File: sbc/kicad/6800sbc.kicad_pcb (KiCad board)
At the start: 2 copper layers, 147 parts, among them J1 AC/DC IN, J10 BAUD RATE, J11 SEGMENT TEST, J12 REG. POWER, J2 5V IN, J3 EXPANSION, J4 LTC, J5 Parallel Port, J6 TX DATA SELECT, J7 RX DATA SELECT, J8 USB POWER, J9 FTDI SERIAL, SW10 "9", SW11 "4", SW12 "5", SW13 "6", SW14 "1", SW15 "2", SW16 "3", SW17 "0", SW18 "RESET", SW2 "D", SW3 "E", SW4 "F", SW5 "A", SW6 "B", SW7 "C", SW8 "7", SW9 "8", U1 LM7805, U10 MAN71A, U11 MAN71A, U12 74LS259, U13 74LS259, U14 74LS259, U15 74LS259, U16 74LS259, U17 74LS259, U18 74LS244, U19 62256 RAM, U2 74LS00, U20 27128, U21 MC6802, U22 ATF16V8B, U23 74LS244, U24 74LS42, U3 74LS04, U4 6821, U5 MC6850, U6 MAN71A, U7 MAN71A, U8 MAN71A, U9 MAN71A, Y1 1.8432 MHz, Y2 3.579545 kHz

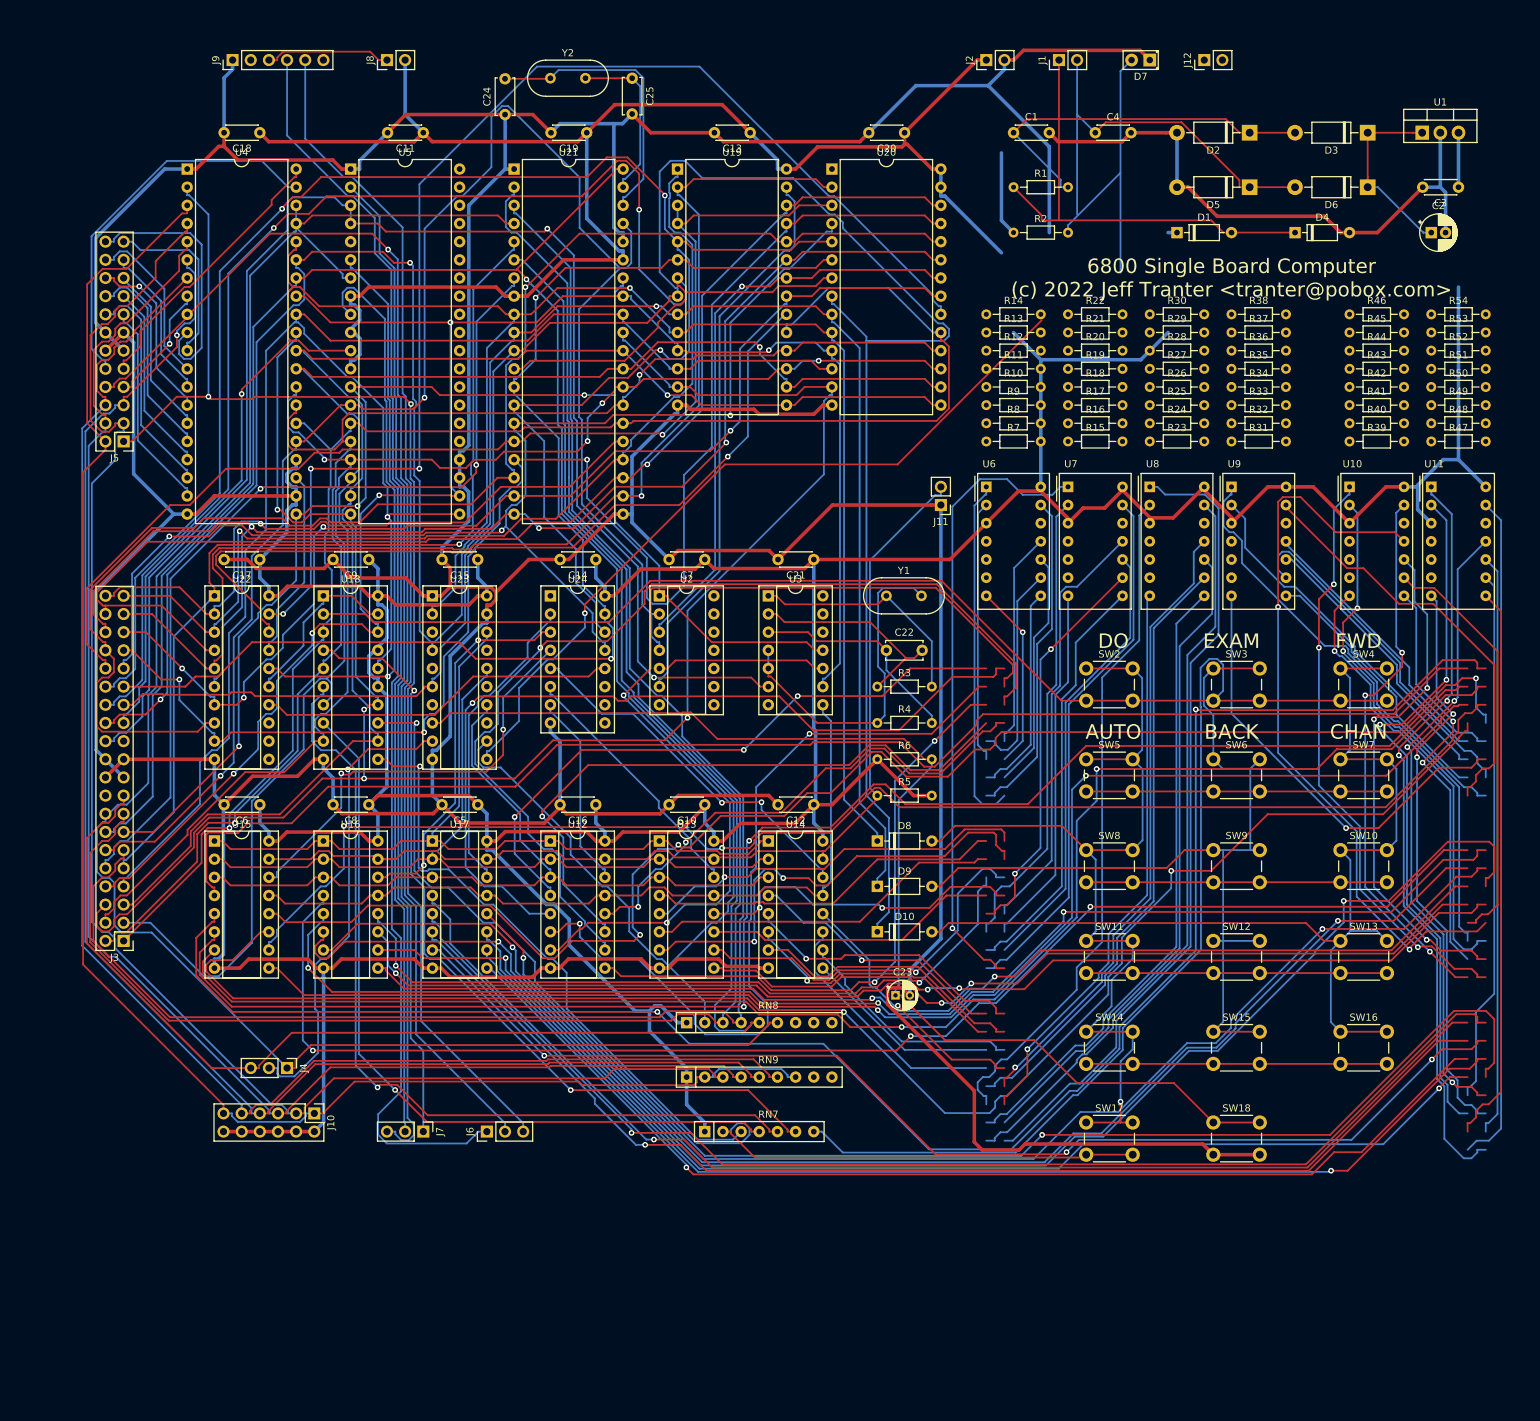
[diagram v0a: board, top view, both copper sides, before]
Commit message: Getting close to ready to order PCBs. Check in all files.
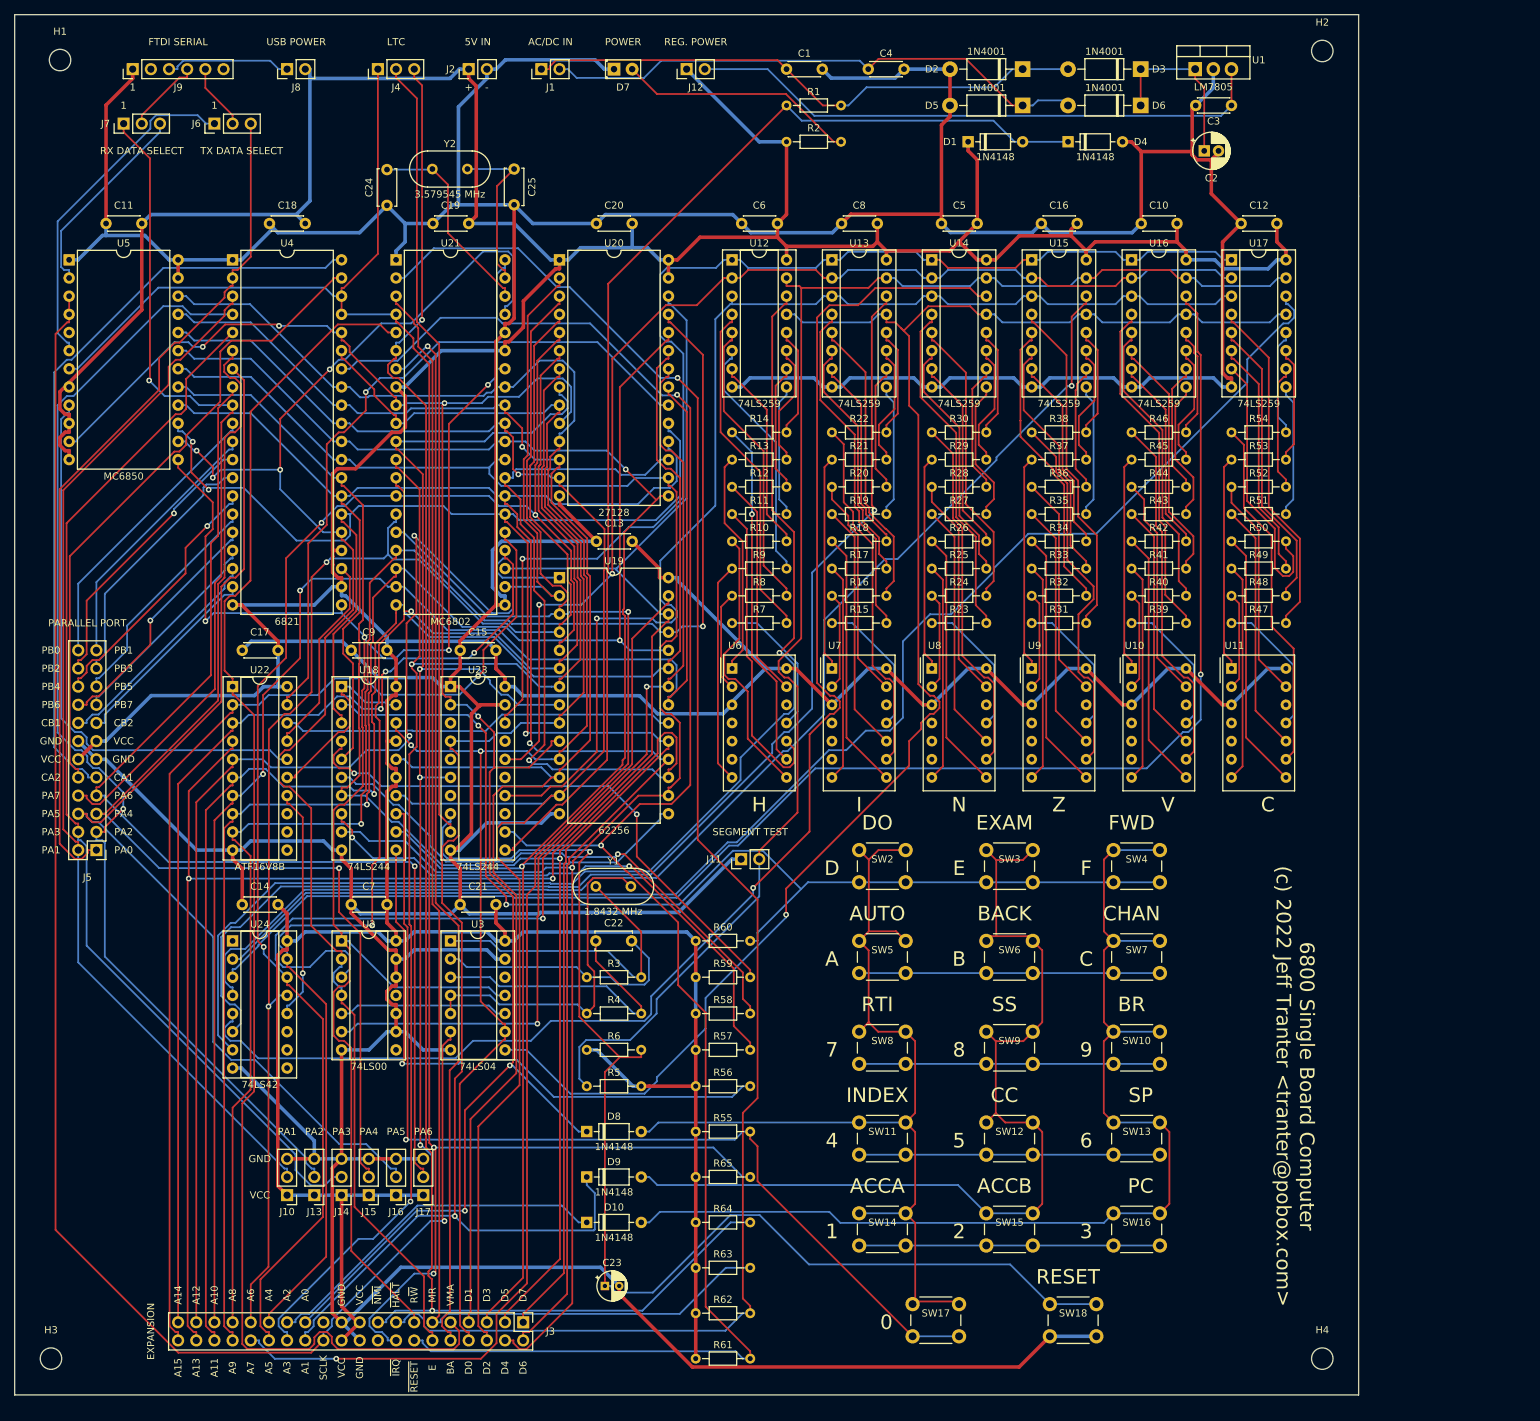
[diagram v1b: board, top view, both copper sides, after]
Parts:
- removed RN7: 8K2, Resistor_THT:R_Array_SIP7
- removed RN8, RN9: 3K, Resistor_THT:R_Array_SIP9
- added H1: MountingHole_3mm, MountingHole:MountingHole_3mm, F.Cu at (39.4, 29.2)
- added H2: MountingHole_3mm, MountingHole:MountingHole_3mm, F.Cu at (215.9, 27.9)
- added H3: MountingHole_3mm, MountingHole:MountingHole_3mm, F.Cu at (38.1, 210.8)
- added H4: MountingHole_3mm, MountingHole:MountingHole_3mm, F.Cu at (215.9, 210.8)
- added J13: PA2, Connector_PinHeader_2.54mm:PinHeader_1x03_P2.54mm_Vertical, F.Cu at (74.9, 188.0)
- added J14: PA3, Connector_PinHeader_2.54mm:PinHeader_1x03_P2.54mm_Vertical, F.Cu at (78.7, 188.0)
- added J15: PA4, Connector_PinHeader_2.54mm:PinHeader_1x03_P2.54mm_Vertical, F.Cu at (82.5, 188.0)
- added J16: PA5, Connector_PinHeader_2.54mm:PinHeader_1x03_P2.54mm_Vertical, F.Cu at (86.4, 188.0)
- added J17: PA6, Connector_PinHeader_2.54mm:PinHeader_1x03_P2.54mm_Vertical, F.Cu at (90.2, 188.0)
- added R55: 8K2, Resistor_THT:R_Axial_DIN0204_L3.6mm_D1.6mm_P7.62mm_Horizontal, F.Cu at (128.3, 179.1)
- added R56: 8K2, Resistor_THT:R_Axial_DIN0204_L3.6mm_D1.6mm_P7.62mm_Horizontal, F.Cu at (128.3, 172.7)
- added R57: 8K2, Resistor_THT:R_Axial_DIN0204_L3.6mm_D1.6mm_P7.62mm_Horizontal, F.Cu at (128.3, 167.6)
- added R58: 8K2, Resistor_THT:R_Axial_DIN0204_L3.6mm_D1.6mm_P7.62mm_Horizontal, F.Cu at (128.3, 162.6)
- added R59: 8K2, Resistor_THT:R_Axial_DIN0204_L3.6mm_D1.6mm_P7.62mm_Horizontal, F.Cu at (128.3, 157.5)
- added R60: 8K2, Resistor_THT:R_Axial_DIN0204_L3.6mm_D1.6mm_P7.62mm_Horizontal, F.Cu at (128.3, 152.4)
- added R61: 3K, Resistor_THT:R_Axial_DIN0204_L3.6mm_D1.6mm_P7.62mm_Horizontal, F.Cu at (128.3, 210.8)
- added R62: 3K, Resistor_THT:R_Axial_DIN0204_L3.6mm_D1.6mm_P7.62mm_Horizontal, F.Cu at (128.3, 204.5)
- added R63: 3K, Resistor_THT:R_Axial_DIN0204_L3.6mm_D1.6mm_P7.62mm_Horizontal, F.Cu at (128.3, 198.1)
- added R64: 3K, Resistor_THT:R_Axial_DIN0204_L3.6mm_D1.6mm_P7.62mm_Horizontal, F.Cu at (128.3, 191.8)
- added R65: 3K, Resistor_THT:R_Axial_DIN0204_L3.6mm_D1.6mm_P7.62mm_Horizontal, F.Cu at (128.3, 185.4)
- J10: value BAUD RATE -> PA1; footprint Connector_PinHeader_2.54mm:PinHeader_2x06_P2.54mm_Vertical -> Connector_PinHeader_2.54mm:PinHeader_1x03_P2.54mm_Vertical
- J5: value Parallel Port -> PARALLEL PORT
- U19: value 62256 RAM -> 62256
- U5: footprint Package_DIP:DIP-40_W15.24mm -> Package_DIP:DIP-24_W15.24mm
- Y2: value 3.579545 kHz -> 3.579545 MHz
- moved J7 147.1 mm to (48.3, 38.1), turned to 90 degrees
- moved J6 146.0 mm to (61.0, 38.1)
- moved J4 140.3 mm to (83.8, 30.5), turned to 90 degrees
- moved U15 140.3 mm to (175.3, 57.1)
- moved U16 139.2 mm to (189.2, 57.1)
- moved U17 138.2 mm to (203.2, 57.1)
- moved C6 108.8 mm to (139.7, 52.1)
- moved C8 108.0 mm to (153.7, 52.1)
- moved C5 107.2 mm to (167.6, 52.1)
- moved C16 105.5 mm to (181.6, 52.1)
- moved C10 104.7 mm to (195.6, 52.1)
- moved C12 103.9 mm to (209.6, 52.1)
- moved U12 85.2 mm to (133.3, 57.1)
- moved U13 84.8 mm to (147.3, 57.1)
- moved U14 84.4 mm to (161.3, 57.1)
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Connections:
- J10 pad 1: PA1 -> VCC
- J10 pad 2: GND -> PA1
- J10 pad 3: PA2 -> GND
- U2 pad 14: (no net) -> VCC
- U2 pad 7: (no net) -> GND
- U3 pad 14: (no net) -> VCC
- U3 pad 7: (no net) -> GND
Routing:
- net Net-(R32-Pad2): track 251.2 -> 41.5 mm, vias 2 -> 0
- net Net-(R37-Pad2): track 225.1 -> 17.2 mm, vias 2 -> 0
- net Net-(R38-Pad2): track 206.7 -> 15.5 mm, vias 3 -> 0
- net Net-(R34-Pad2): track 216.9 -> 27.5 mm, vias 2 -> 0
- net Net-(R33-Pad2): track 220.2 -> 34.7 mm, vias 2 -> 0
- net Net-(R35-Pad2): track 199.2 -> 18.6 mm, vias 2 -> 0
- net Net-(R44-Pad2): track 196.9 -> 18.3 mm, vias 2 -> 0
- net Net-(R36-Pad2): track 196.2 -> 17.9 mm, vias 3 -> 0
- net Net-(R42-Pad2): track 197.2 -> 27.4 mm, vias 2 -> 0
- net Net-(R41-Pad2): track 197.6 -> 34.7 mm, vias 2 -> 0
- net Net-(R54-Pad2): track 174.6 -> 15.1 mm, vias 2 -> 0
- net ~DISP5EN: track 52.3 -> 211.5 mm, vias 2 -> 1
- net ~DISP6EN: track 43.3 -> 198.0 mm
- net Net-(J6-Pad2): track 162.8 -> 9.20 mm
- net Net-(R46-Pad2): track 169.0 -> 15.5 mm, vias 3 -> 0
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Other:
- board outline added: 188 x 193 mm
- board text added: "+"
- board text added: "-"
- board text added: "0"
- board text added: "1"
- board text added: "2"
- board text added: "3"
- board text added: "4"
- board text added: "5"
- board text added: "6"
- board text added: "7"
- board text added: "8"
- board text added: "9"
- board text added: "A"
- board text added: "A0"
- board text added: "A1"
- board text added: "A10"
- board text added: "A11"
- board text added: "A12"
- board text added: "A13"
- board text added: "A14"
- board text added: "A15"
- board text added: "A2"
- board text added: "A3"
- board text added: "A4"
- board text added: "A5"
- board text added: "A6"
- board text added: "A7"
- board text added: "A8"
- board text added: "A9"
- board text added: "ACCA"
- board text added: "ACCB"
- board text added: "B"
- board text added: "BA"
- board text added: "BR"
- board text added: "C"
- board text added: "CA1"
- board text added: "CA2"
- board text added: "CB1"
- board text added: "CB2"
- board text added: "CC"
- board text added: "D"
- board text added: "D0"
- board text added: "D1"
- board text added: "D2"
- board text added: "D3"
- board text added: "D4"
- board text added: "D5"
- board text added: "D6"
- board text added: "D7"
- board text added: "E"
- board text added: "F"
- board text added: "GND"
- board text added: "H"
- board text added: "I"
- board text added: "INDEX"
- board text added: "MR"
- board text added: "N"
- board text added: "PA0"
- board text added: "PA1"
- board text added: "PA2"
- board text added: "PA3"
- board text added: "PA4"
- board text added: "PA5"
- board text added: "PA6"
- board text added: "PA7"
- board text added: "PB0"
- board text added: "PB1"
- board text added: "PB2"
- board text added: "PB3"
- board text added: "PB4"
- board text added: "PB5"
- board text added: "PB6"
- board text added: "PB7"
- board text added: "PC"
- board text added: "RESET"
- board text added: "RTI"
- board text added: "R~W"
- board text added: "SCLK"
- board text added: "SP"
- board text added: "SS"
- board text added: "V"
- board text added: "VCC"
- board text added: "VMA"
- board text added: "Z"
- board text added: "~HALT"
- board text added: "~IRQ"
- board text added: "~NMI"
- board text added: "~RESET"

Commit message: Optimizing board layout.
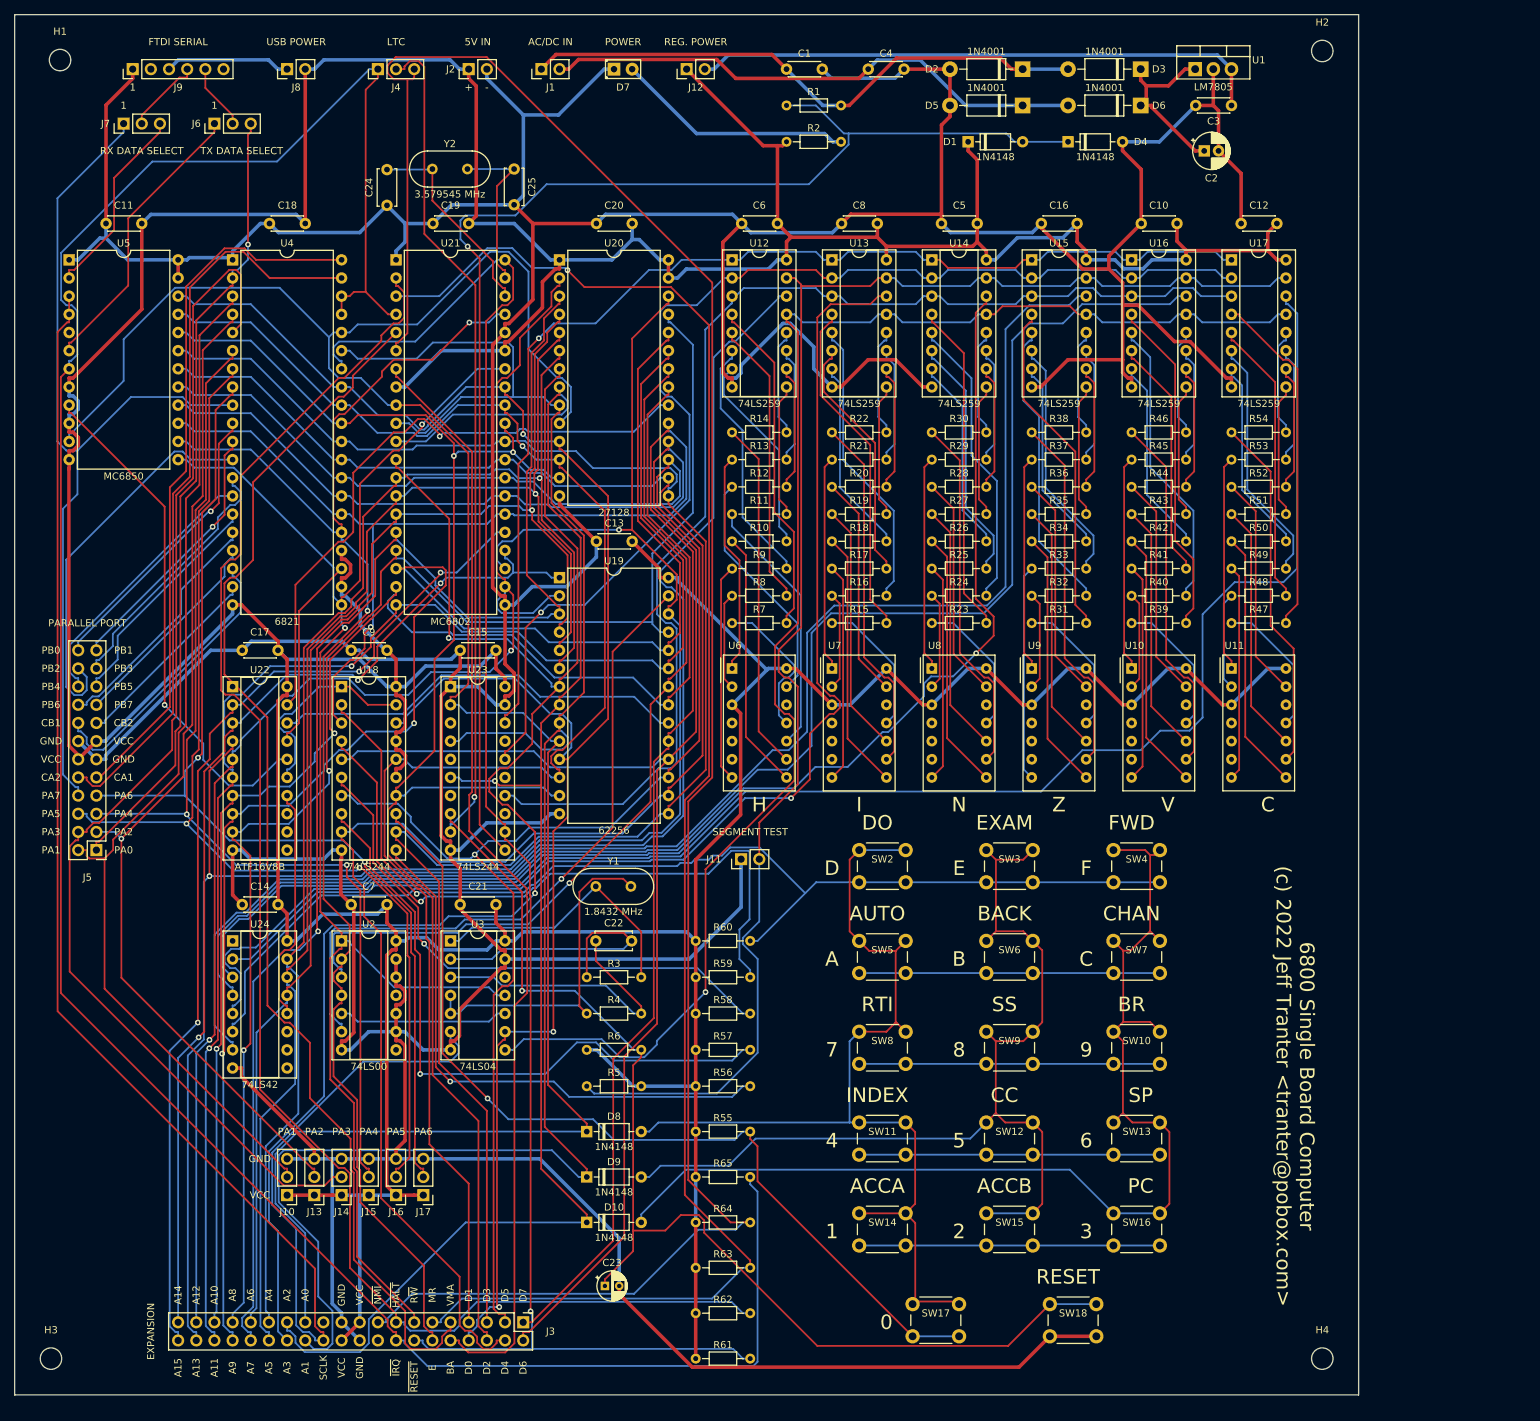
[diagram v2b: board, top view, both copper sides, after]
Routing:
- net ~IRQ: track 287.5 -> 351.5 mm, vias 2 -> 0
- net ~NMI: track 238.0 -> 300.3 mm, vias 2 -> 0
- net A0: track 268.5 -> 321.2 mm, vias 6 -> 0
- net A1: track 230.7 -> 274.8 mm, vias 1 -> 0
- net MR: track 194.3 -> 235.9 mm, vias 0 -> 1
- net D5: track 299.0 -> 258.7 mm, vias 2 -> 1
- net ~RESET: track 277.7 -> 238.7 mm, vias 2 -> 1
- net GND: track 994.3 -> 1027.5 mm
- net A7: track 234.2 -> 202.4 mm, vias 2 -> 1
- net 60HZ: track 163.1 -> 192.4 mm, vias 0 -> 1
- net VCC: track 931.5 -> 960.4 mm
- net VMA: track 198.2 -> 173.1 mm
- net R~W: track 239.0 -> 214.1 mm, vias 4 -> 2
- net PA3: track 148.7 -> 170.1 mm
- net ~READ: track 146.6 -> 125.4 mm, vias 2 -> 1
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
